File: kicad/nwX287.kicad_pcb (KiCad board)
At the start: 2 copper layers, 18.3 x 31.1 mm, 4 parts, among them U1 bq4285, U2 socket, Y1 32.768kHz 6pF

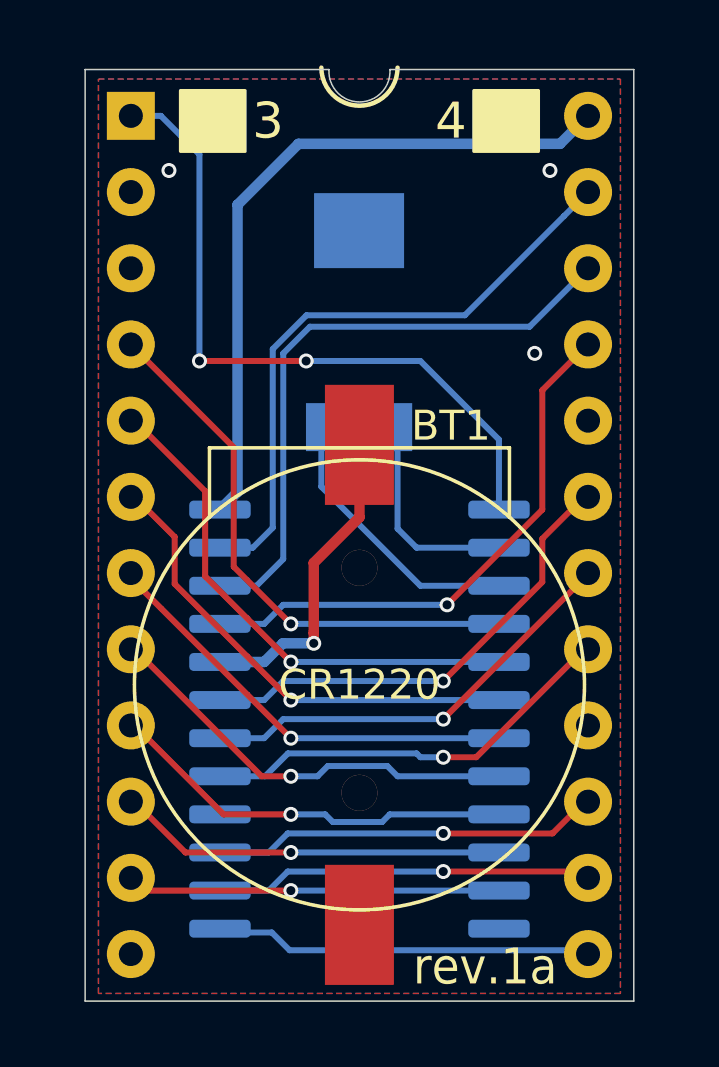
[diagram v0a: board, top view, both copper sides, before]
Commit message: CR2032, SSOP-24 and MOT
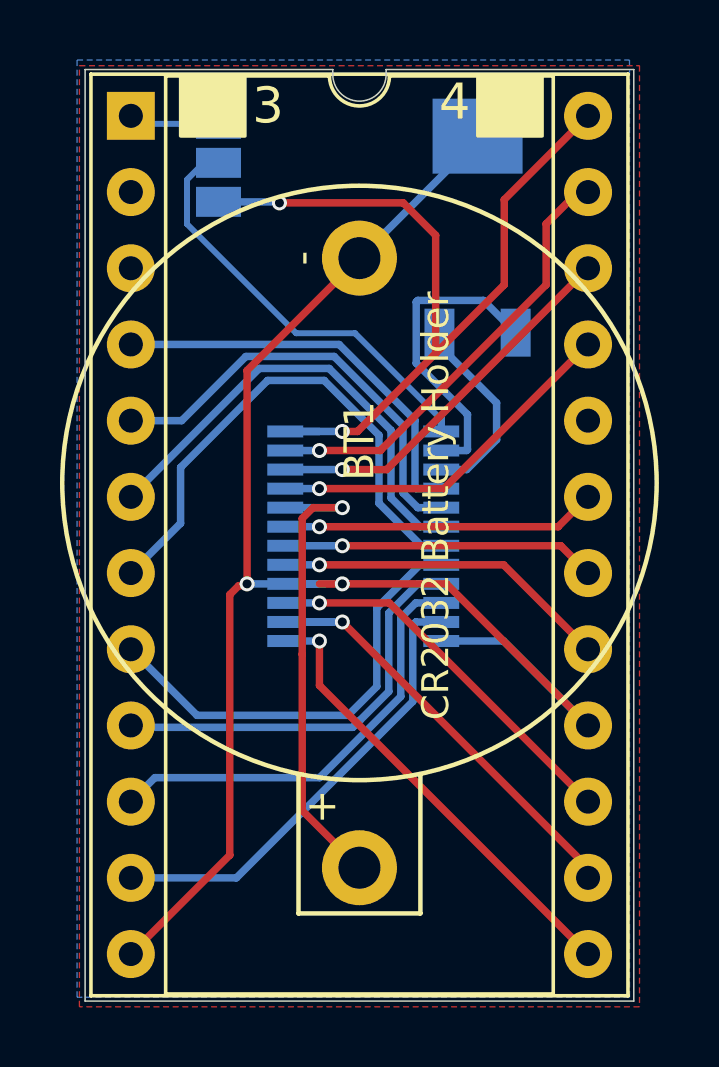
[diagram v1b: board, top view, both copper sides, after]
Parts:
- added J1: Conn_01x03_Male, Jumper:SolderJumper-3_P1.3mm_Open_Pad1.0x1.5mm_NumberLabels, B.Cu at (129.9, 81.0)
- BT1: value CR1220 -> CR2032; footprint nwX287:BatteryHolder_CR1220 -> nwX287.2032.ssop:CR2032_battery_holder
- U1: footprint Package_SO:SOIC-24W_7.5x15.4mm_P1.27mm -> Package_SO:SSOP-24_3.9x8.7mm_P0.635mm
- moved U1 6.10 mm to (134.7, 93.5)
- moved BT1 6.10 mm to (134.6, 104.5), turned to 90 degrees
- moved Y1 5.05 mm to (138.6, 83.2)
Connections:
- U1 pad 1: VOUT -> Net-(J1-Pad2)
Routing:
- net GND: track 0.00 -> 53.7 mm, vias 3 -> 2
- net VOUT: track 23.1 -> 3.55 mm, vias 2 -> 0
- net Net-(J1-Pad2): track 0.00 -> 14.8 mm
- net CEO: track 20.7 -> 13.3 mm, vias 0 -> 1
- net CEI: track 18.5 -> 12.1 mm
- net SQW: track 20.7 -> 14.9 mm, vias 0 -> 1
- net VCC: track 23.3 -> 28.9 mm, vias 0 -> 2
- net INT: track 16.0 -> 10.5 mm
- net BC: track 10.6 -> 15.9 mm
- net AD0: track 18.5 -> 13.7 mm, vias 1 -> 0
- net RST: track 14.7 -> 10.6 mm
- net X1: track 6.86 -> 10.3 mm
- net AD3: track 14.8 -> 17.7 mm, vias 1 -> 0
- net DS: track 14.2 -> 11.3 mm
- net AS: track 12.6 -> 15.5 mm
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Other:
- outline, holes or cut-outs redrawn
- board text added: "1-2 2-3"
- board text added: "1-2 N/A"
- board text added: "2"
- board text added: "24-SSOP"
- board text added: "3287"
- board text added: "4287"
- board text added: "CR2032 Battery Holder"
- board text added: "Intel Motorola"
- board text added: "J1(MOT)"
- board text added: "by Necroware 2032 SSOP by Scrap Computing"
- board text added: "by Necroware CR2032 SSOP MOT by Scrap Computing"
- board text added: "nwX287.2032.ssop.mot"
- board text added: "rev.1a.2032.ssop.mot"
- board text removed: "by Necroware"
- board text removed: "nwX287"
- board text removed: "rev.1a"
